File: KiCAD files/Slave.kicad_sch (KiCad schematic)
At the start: 11 parts, among them U5 NUCLEO64-F446RE

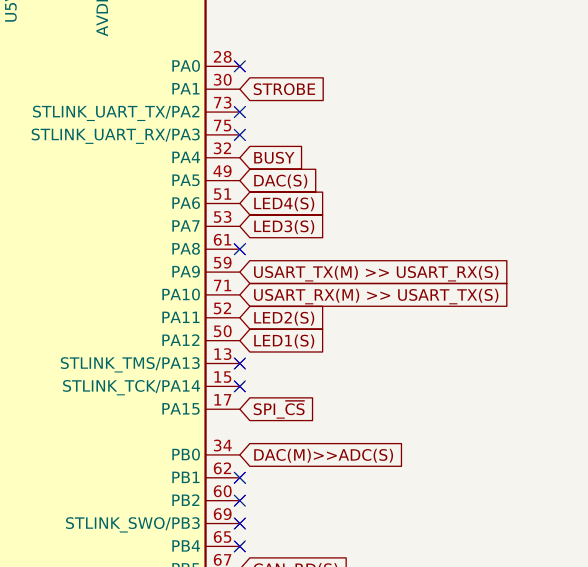
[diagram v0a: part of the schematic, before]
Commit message: update
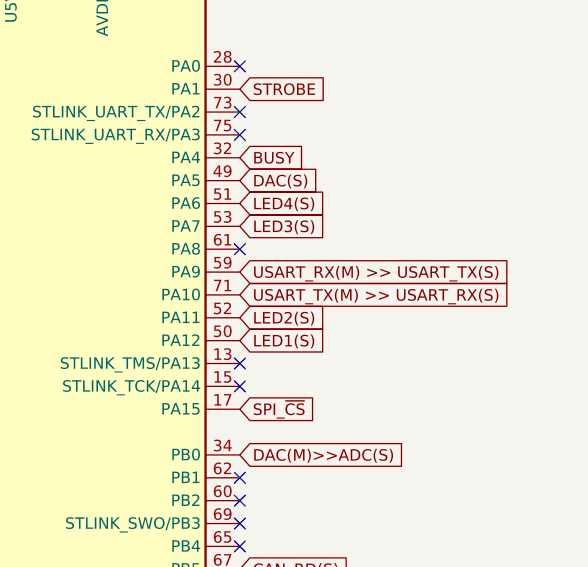
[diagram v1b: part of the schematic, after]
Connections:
- net USART_RX(M) >> USART_TX(S): now also U5.59 (PA9); no longer U5.71 (PA10)
- net USART_TX(M) >> USART_RX(S): now also U5.71 (PA10); no longer U5.59 (PA9)
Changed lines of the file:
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@@
     )
   )
-  (global_label "USART_TX(M) >> USART_RX(S)" (shape input) (at 172.72 78.74 0) (fields_autoplaced)
+  (global_label "USART_TX(M) >> USART_RX(S)" (shape input) (at 172.72 81.28 0) (fields_autoplaced)
     (effects (font (size 1.27 1.27)) (justify left))
-    (property "Intersheetrefs" "${INTERSHEET_REFS}" (at 205.1571 78.74 0)
+    (property "Intersheetrefs" "${INTERSHEET_REFS}" (at 205.1571 81.28 0)
       (effects (font (size 1.27 1.27)) (justify left) hide)
     )
@@
     )
   )
-  (global_label "USART_RX(M) >> USART_TX(S)" (shape input) (at 172.72 81.28 0) (fields_autoplaced)
+  (global_label "USART_RX(M) >> USART_TX(S)" (shape input) (at 172.72 78.74 0) (fields_autoplaced)
     (effects (font (size 1.27 1.27)) (justify left))
-    (property "Intersheetrefs" "${INTERSHEET_REFS}" (at 205.1571 81.28 0)
+    (property "Intersheetrefs" "${INTERSHEET_REFS}" (at 205.1571 78.74 0)
       (effects (font (size 1.27 1.27)) (justify left) hide)
     )
